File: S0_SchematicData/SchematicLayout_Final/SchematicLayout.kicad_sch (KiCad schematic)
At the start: 9 parts, among them P1 Conn_Plug_2P, Q4 Auerbach_R, Q5 Auerbach_G, Q6 Auerbach_B, U1 LMZM23600V5, U2 ESP32-WROOM-32D

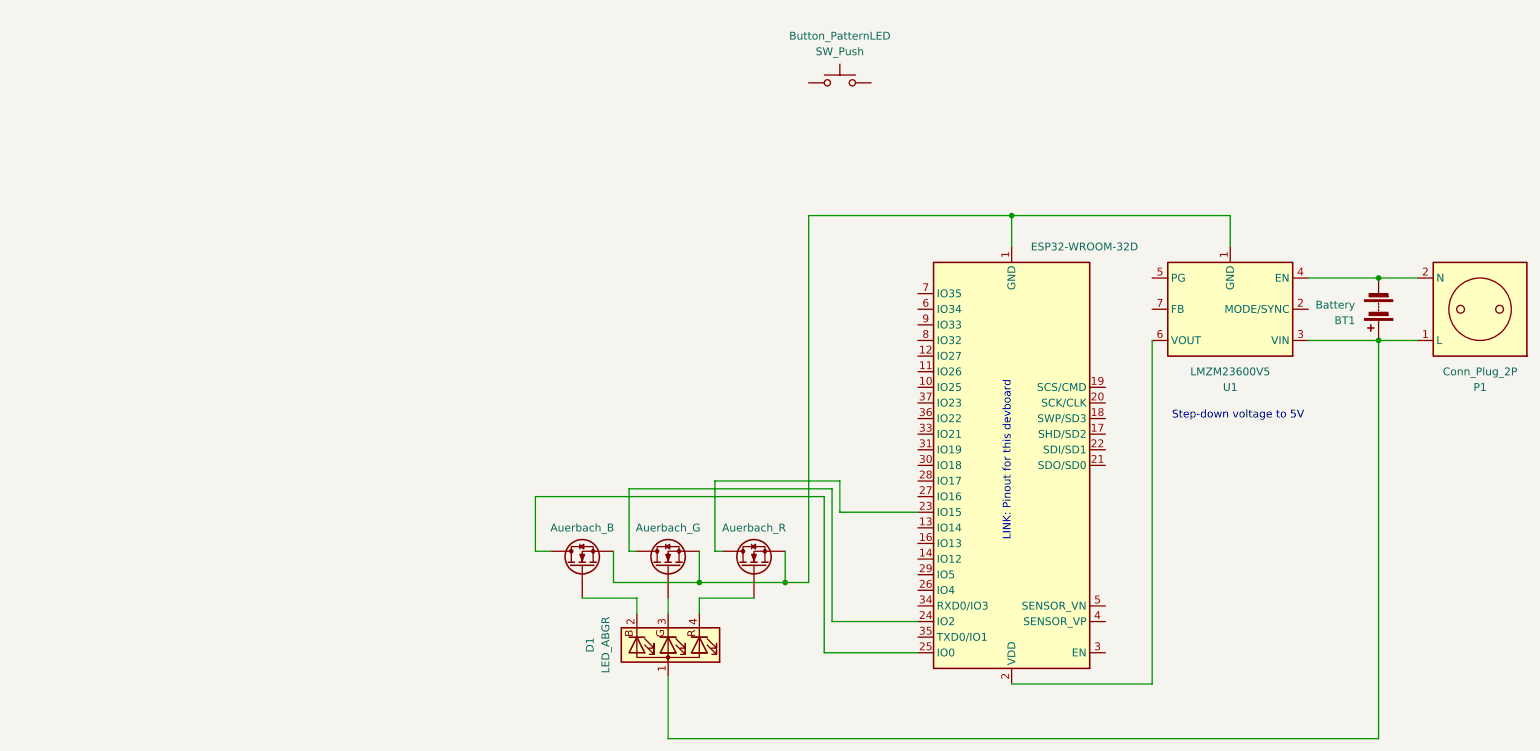
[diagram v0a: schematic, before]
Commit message: Completion of schematic
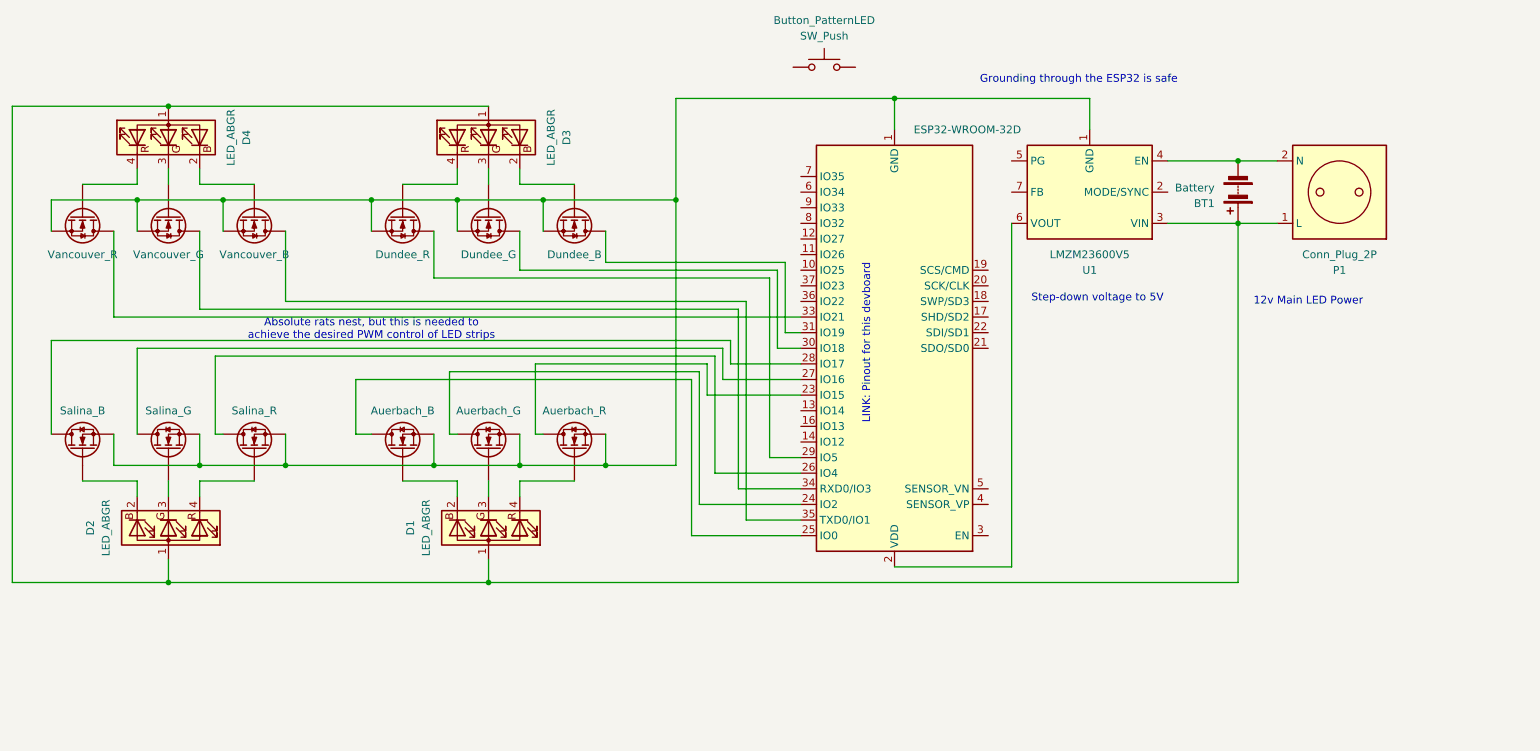
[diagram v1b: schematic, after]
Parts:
- added D2, D3, D4: LED_ABGR, symbol Device:LED_ABGR
- added Q10: Dundee_B, symbol Device:Q_NMOS
- added Q11: Dundee_G, symbol Device:Q_NMOS
- added Q12: Dundee_R, symbol Device:Q_NMOS
- added Q13: Vancouver_R, symbol Device:Q_NMOS
- added Q14: Vancouver_G, symbol Device:Q_NMOS
- added Q15: Vancouver_B, symbol Device:Q_NMOS
- added Q7: Salina_B, symbol Device:Q_NMOS
- added Q8: Salina_G, symbol Device:Q_NMOS
- added Q9: Salina_R, symbol Device:Q_NMOS
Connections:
- net at Q4.S, Q5.S, Q6.S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: now also Q10.S, Q11.S, Q12.S, Q13.S, Q14.S, Q15.S, Q7.S, Q8.S, Q9.S
- net at BT1.1 (+), D1.1 (A), P1.1 (L)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: now also D2.1 (A), D3.1 (A), D4.1 (A)
- net at U2.26 (IO4): now also Q9.D
- net at U2.27 (IO16): now also Q8.D
- net at U2.28 (IO17): now also Q7.D
- net at U2.29 (IO5): now also Q12.D
- net at U2.30 (IO18): now also Q11.D
- net at U2.31 (IO19): now also Q10.D
- net at U2.33 (IO21): now also Q13.D
- net at U2.34 (RXD0/IO3): now also Q14.D
- net at U2.35 (TXD0/IO1): now also Q15.D
- new net: D2.4 (RK), Q9.G
- new net: D4.2 (BK), Q15.G
- new net: D4.3 (GK), Q14.G
- new net: D4.4 (RK), Q13.G
- new net: D3.3 (GK), Q11.G
- new net: D3.2 (BK), Q10.G
- new net: D2.2 (BK), Q7.G
- new net: D2.3 (GK), Q8.G
- new net: D3.4 (RK), Q12.G
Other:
- note added: "12v Main LED Power"
- note added: "Absolute rats nest, but this is needed to achieve the desired PWM control of LED strips"
- note added: "Grounding through the ESP32 is safe"
- moved on the sheet: BT1, Button_PatternLED, D1, P1, U1
